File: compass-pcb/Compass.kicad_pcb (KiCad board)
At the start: 2 copper layers, 9 parts

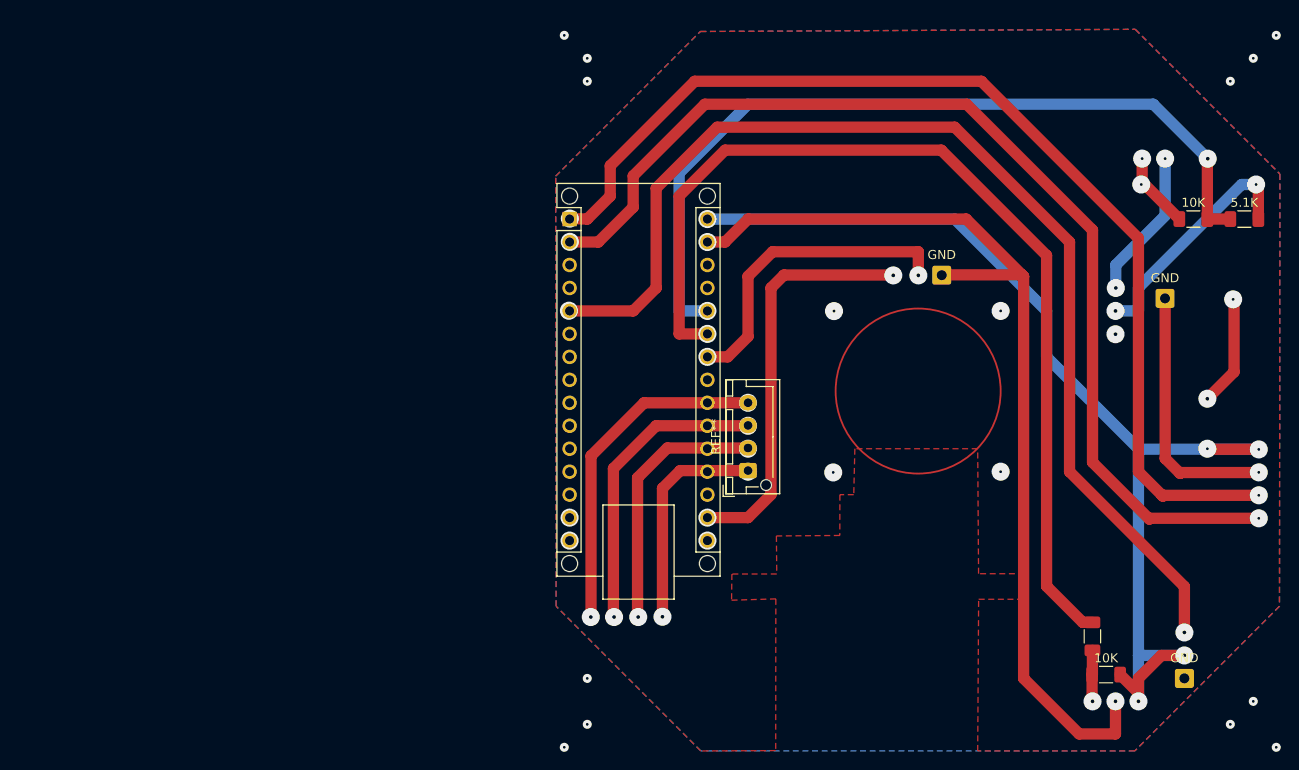
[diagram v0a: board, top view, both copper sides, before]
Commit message: comments for anchors
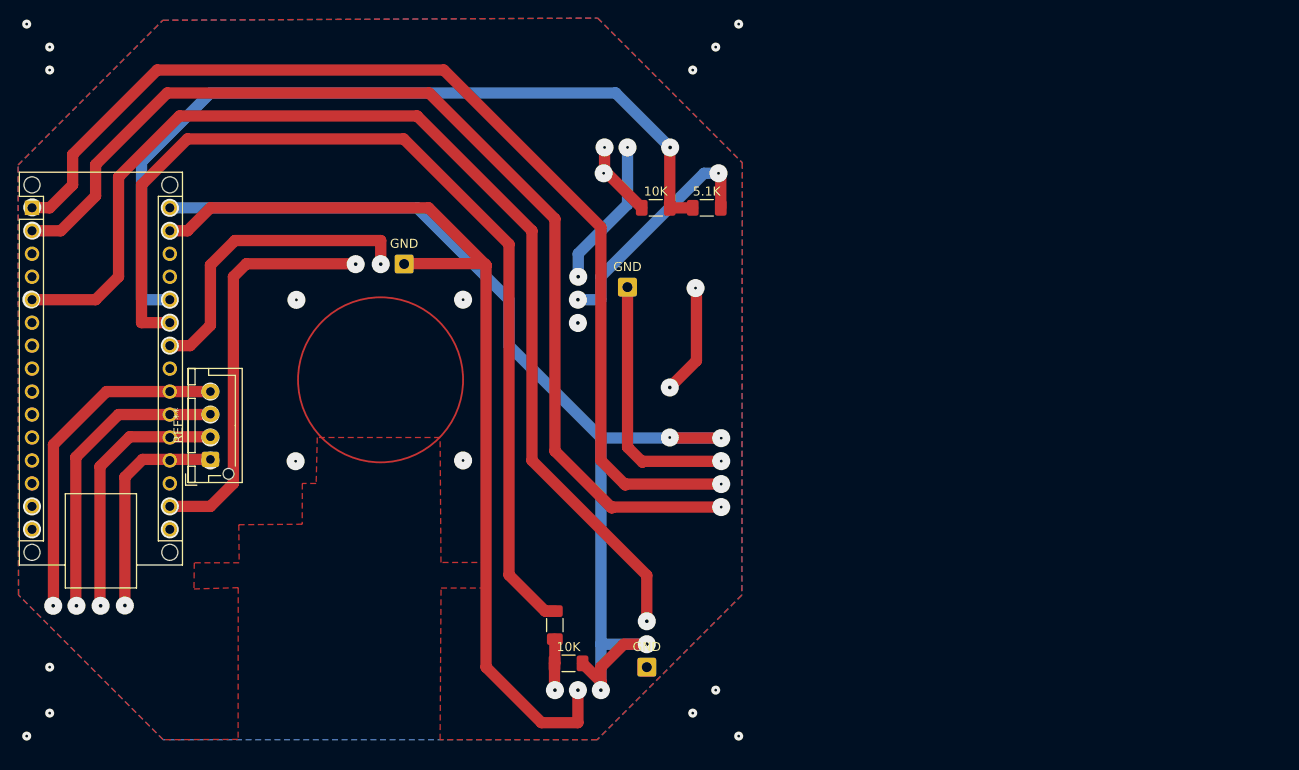
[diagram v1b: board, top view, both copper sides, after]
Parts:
- moved 10K 59.5 mm to (168.1, 125.3)
- moved 10K 59.5 mm to (177.8, 75.0)
- moved 5.1K 59.5 mm to (166.6, 121.1)
- moved 5.1K 59.5 mm to (183.4, 75.0)
- moved GND 59.5 mm to (174.6, 83.7)
- moved GND 59.5 mm to (149.9, 81.2)
- moved GND 59.5 mm to (176.8, 125.8)
- moved REF** 59.5 mm to (128.5, 102.8)
- moved REF** 59.5 mm to (108.8, 75.0)
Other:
- board text added: "Alignment anchors: 1) print stencil 2) drill these holes 3) align back side stencil by these holes"
